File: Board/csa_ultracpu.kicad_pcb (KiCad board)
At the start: 4 copper layers, 160 x 100.1 mm, 175 parts, among them IC13 74244DW, IC14 74LVC14, IC16 74LVC8T245SO24, IC18 74LVC06, IC19 74244DW, IC2 74HCT245DW, IC3 74LVC125, IC4 74HCT245DW, IC5 74HCT245DW, IC6 741G04DBV, IC7 74LVC138, IC8 MAX3421E, P1 CSABUS, Q2 32kHz, Q3 12MHz, U1 IS61C5128AL-10TLI, U2 IS61C5128AL-10TLI, X1 SJ1-3513N, X2 D-SUB15-HDR15RA, X3 SG-8002CE

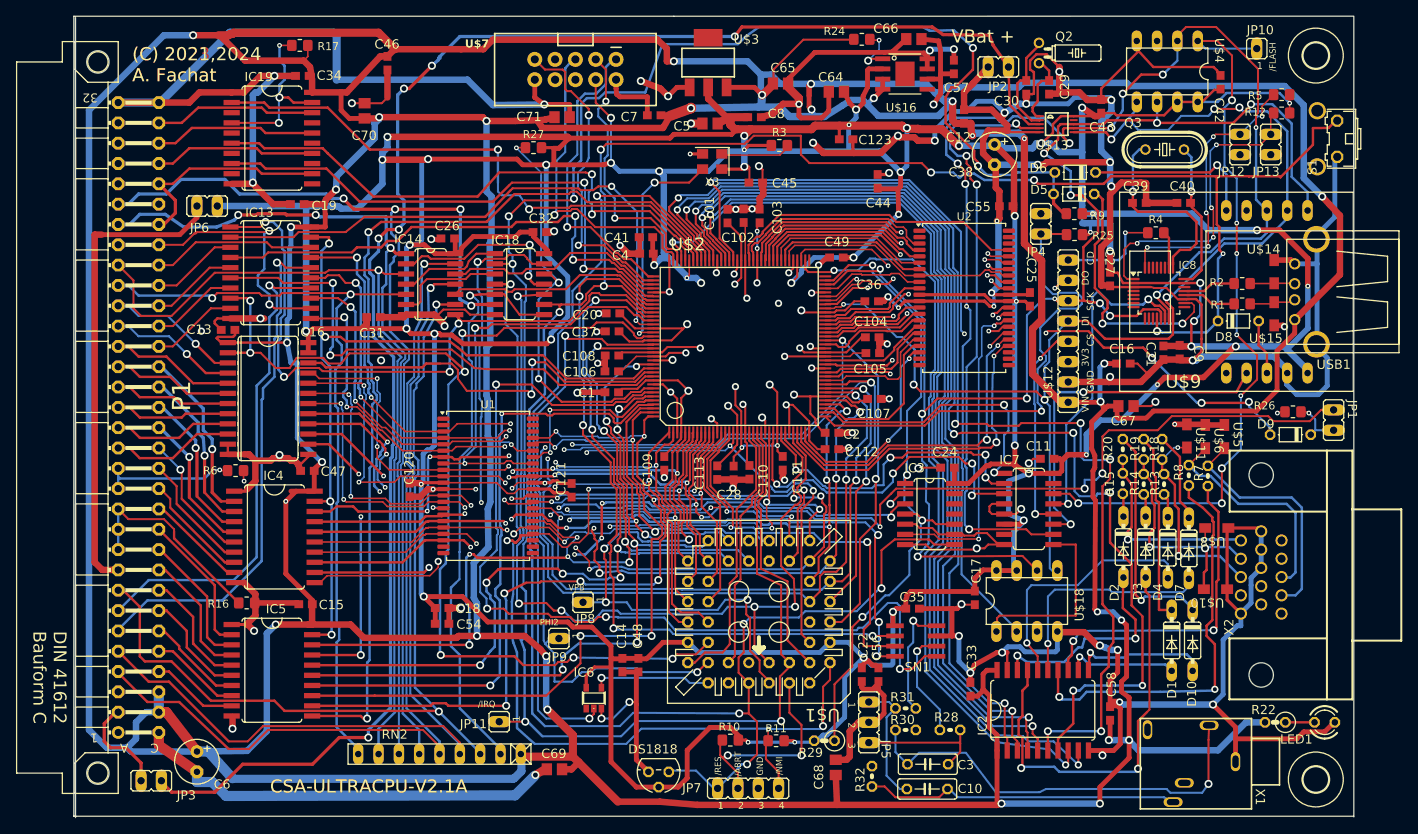
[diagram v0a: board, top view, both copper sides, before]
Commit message: more work on r2.1a - only bom xls is missing/outdated
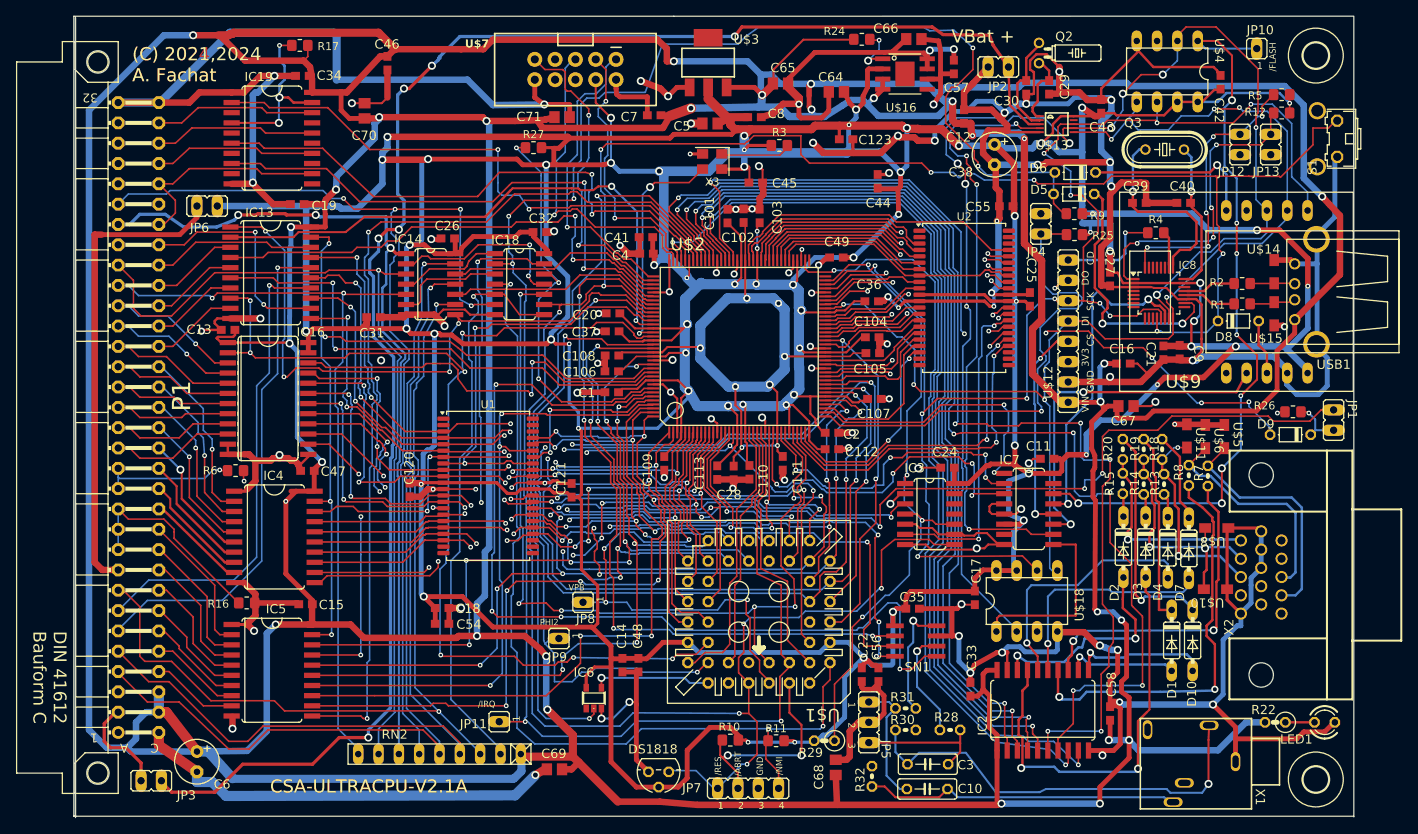
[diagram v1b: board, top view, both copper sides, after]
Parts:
- C121: value 1u -> 0.1u
- C9: value 1.0u Cer -> 1u
- D9: value 1N4148 -> 1N4448
- USB1: value (none) -> USB-A-H
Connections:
- U$2 pad 67: SPI_IN3 -> RAMD0
- U$2 pad 69: RAMD0 -> RAMD7
- U$2 pad 75: RAMD7 -> SPI_IN3
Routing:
- net V33: track 1120.9 -> 1171.5 mm, vias 64 -> 65
- net GND: track 950.8 -> 941.5 mm
- net SPI_IN3: track 32.1 -> 37.3 mm
- net VCC: track 1024.4 -> 1019.5 mm
- net RAMD7: track 29.0 -> 24.5 mm
- net A14: track 122.1 -> 119.8 mm
- net /BUS I/O/BR/-W: track 30.5 -> 28.3 mm
- net /LDAC: track 118.8 -> 116.6 mm
- net BE_IN: track 83.1 -> 80.9 mm
- net /BUS I/O//BNMI: track 97.6 -> 95.5 mm
- net /IRQ: track 255.5 -> 253.6 mm
- net R/-W: track 148.2 -> 146.3 mm
- net A12: track 115.1 -> 113.2 mm
- net /A/V Out/IBLUE: track 29.5 -> 27.6 mm
- net SPI_MOSI: track 152.0 -> 150.1 mm
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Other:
- board text added: "(C) 2024 A. Fachat"
- board text removed: "(C) 2023 A. Fachat"
